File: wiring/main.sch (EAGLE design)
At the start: 38 parts, among them IC1 attiny 2313A, J2 J7MM, J3 J5MM, J4 J10MM, J5 J7MM, J6 J5MM, J7 J5MM, Q1 12MHz, T1 BD433, X1 USB-B

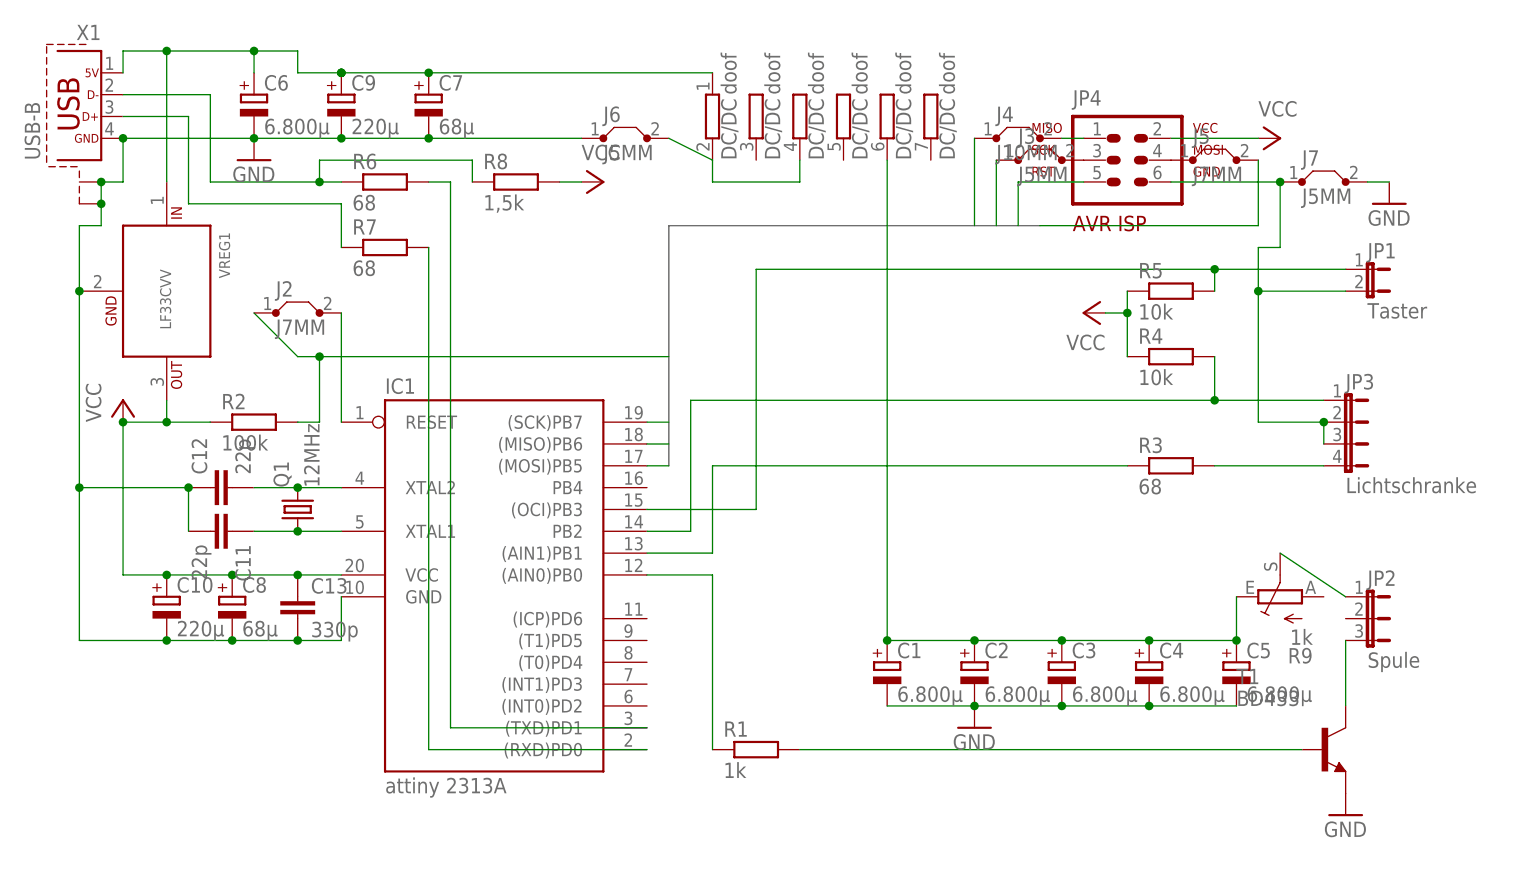
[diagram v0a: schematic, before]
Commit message: ändern auf mosfet
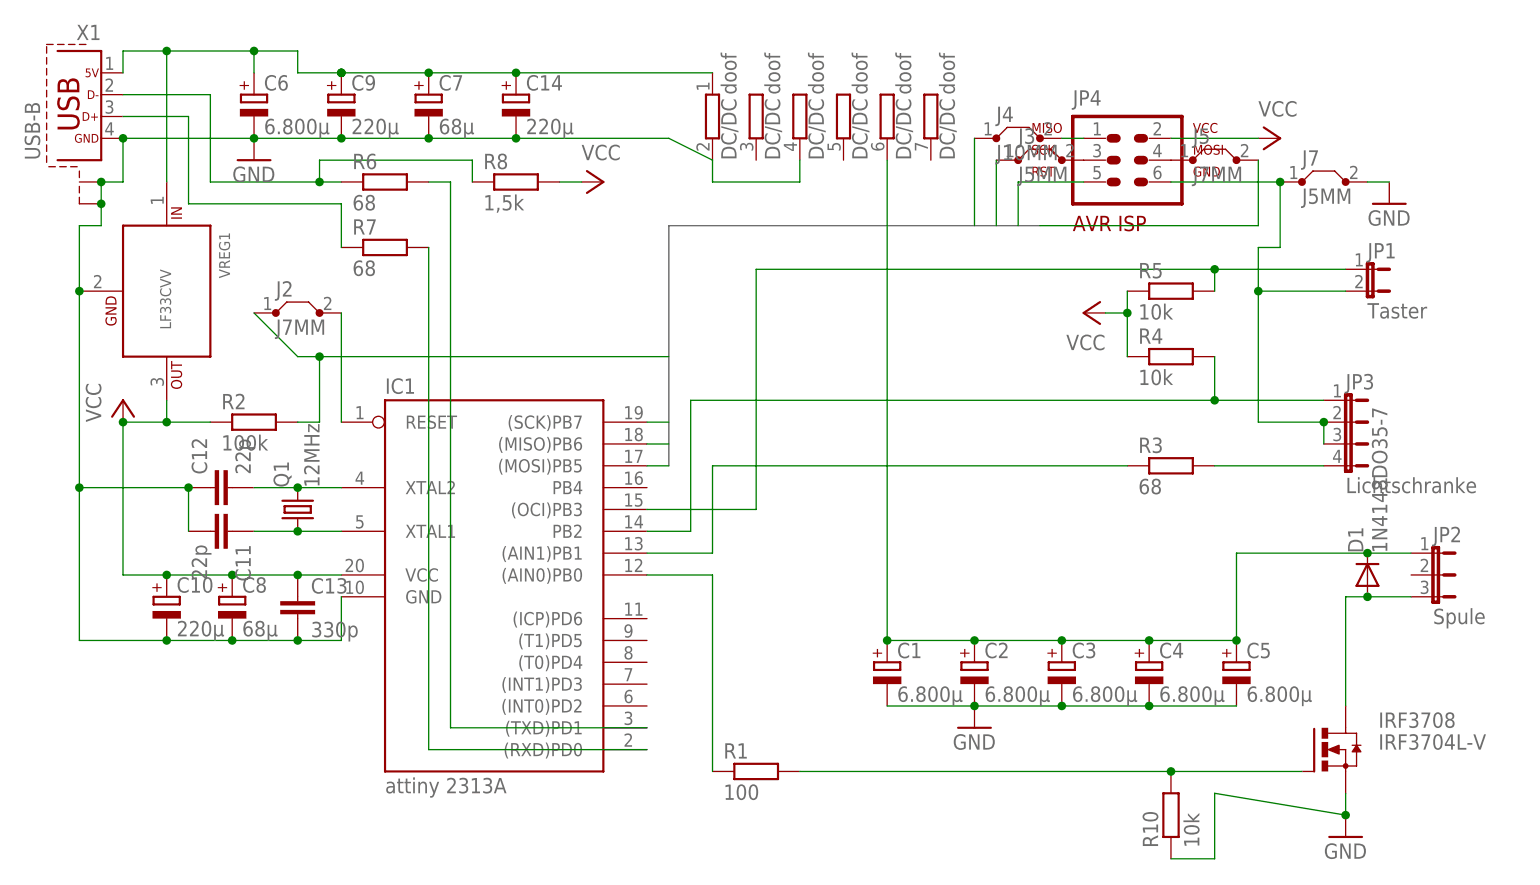
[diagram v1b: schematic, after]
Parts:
- removed J6: J5MM, jumper:J5MM
- removed R9: 1k, pot:TRIM_EU-PT10
- removed T1: BD433, transistor:BD239
- added C14: 220µ, resistor:CPOL-EUE2.5-7
- added D1: 1N4148DO35-7, diode:1N4148DO35-7
- added IRF3708: IRF3704L-V, transistor-power:IRF3704L-V
- added R10: 10k, rcl:R-EU_0207/10
- R1: value 1k -> 100
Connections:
- removed net N$21: DC/DCA.2, DC/DCC.2, J6.2
- removed net N$5: JP2.1, R9.S
- net 5V: now also C14.+
- net GND: now also C14.-, DC/DCA.2, DC/DCC.2, IRF3708.S, R10.1; no longer J6.1, T1.E
- net N$2: now also IRF3708.G, R10.2; no longer T1.B
- net N$3: now also D1.A, IRF3708.D; no longer T1.C
- net N$4: now also D1.C, JP2.1; no longer R9.E
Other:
- moved on the sheet: JP2, R1
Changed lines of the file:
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@@
 <part name="C9" library="resistor" deviceset="CPOL-EU" device="E2.5-7" value="220µ"/>
 <part name="C10" library="resistor" deviceset="CPOL-EU" device="E2.5-7" value="220µ"/>
-<part name="T1" library="transistor" deviceset="BD239" device="" value="BD433"/>
-<part name="R1" library="rcl" deviceset="R-EU_" device="0207/10" value="1k"/>
+<part name="R1" library="rcl" deviceset="R-EU_" device="0207/10" value="100"/>
 <part name="DC/DC" library="resistor-sil" deviceset="GE06RP" device="" value="doof"/>
 <part name="R2" library="rcl" deviceset="R-EU_" device="0207/10" value="100k"/>
@@
 <part name="P+1" library="supply1" deviceset="VCC" device=""/>
 <part name="GND6" library="supply1" deviceset="GND" device=""/>
-<part name="R9" library="pot" deviceset="TRIM_EU-" device="PT10" value="1k"/>
 <part name="J2" library="jumper" deviceset="J" device="7MM" value="J7MM"/>
 <part name="GND7" library="supply1" deviceset="GND" device=""/>
@@
 <part name="J4" library="jumper" deviceset="J" device="10MM"/>
 <part name="J5" library="jumper" deviceset="J" device="7MM" value="J7MM"/>
-<part name="J6" library="jumper" deviceset="J" device="5MM"/>
 <part name="GND4" library="supply1" deviceset="GND" device=""/>
 <part name="J7" library="jumper" deviceset="J" device="5MM"/>
 <part name="GND3" library="supply1" deviceset="GND" device=""/>
+<part name="D1" library="diode" deviceset="1N4148" device="DO35-7"/>
+<part name="IRF3708" library="transistor-power" deviceset="IRF3704" device="L-V"/>
+<part name="R10" library="rcl" deviceset="R-EU_" device="0207/10" value="10k"/>
+<part name="C14" library="resistor" deviceset="CPOL-EU" device="E2.5-7" value="220µ"/>
 </parts>
 <sheets>
@@
 <instance part="IC1" gate="G$1" x="25.4" y="33.02"/>
 <instance part="JP1" gate="A" x="127" y="71.12" rot="R270"/>
-<instance part="JP2" gate="1" x="127" y="30.48" rot="R270"/>
+<instance part="JP2" gate="1" x="134.62" y="35.56" rot="R270"/>
 <instance part="JP3" gate="G$1" x="124.46" y="53.34" rot="R270"/>
 <instance part="C1" gate="G$1" x="71.12" y="25.4"/>
@@
 <instance part="C9" gate="G$1" x="7.62" y="91.44"/>
 <instance part="C10" gate="G$1" x="-12.7" y="33.02"/>
-<instance part="T1" gate="G$1" x="121.92" y="15.24"/>
-<instance part="R1" gate="G$1" x="55.88" y="15.24"/>
+<instance part="R1" gate="G$1" x="55.88" y="12.7"/>
 <instance part="DC/DC" gate="A" x="50.8" y="88.9"/>
 <instance part="DC/DC" gate="B" x="55.88" y="88.9"/>
@@
 <instance part="P+4" gate="VCC" x="116.84" y="86.36" rot="R270"/>
 <instance part="P+1" gate="VCC" x="-17.78" y="55.88"/>
-<instance part="GND6" gate="1" x="124.46" y="7.62"/>
-<instance part="R9" gate="1" x="116.84" y="33.02" rot="R90"/>
+<instance part="GND6" gate="1" x="124.46" y="5.08"/>
 <instance part="J2" gate="1" x="2.54" y="66.04"/>
 <instance part="GND7" gate="1" x="129.54" y="78.74"/>
@@
 <instance part="J4" gate="1" x="86.36" y="86.36"/>
 <instance part="J5" gate="1" x="109.22" y="83.82"/>
-<instance part="J6" gate="1" x="40.64" y="86.36"/>
 <instance part="GND4" gate="1" x="81.28" y="17.78"/>
 <instance part="J7" gate="1" x="121.92" y="81.28"/>
 <instance part="GND3" gate="1" x="-2.54" y="83.82"/>
+<instance part="D1" gate="G$1" x="127" y="35.56" rot="R90"/>
+<instance part="IRF3708" gate="G$1" x="121.92" y="15.24"/>
+<instance part="R10" gate="G$1" x="104.14" y="7.62" rot="R90"/>
+<instance part="C14" gate="G$1" x="27.94" y="91.44"/>
 </instances>
 <busses>
@@
 <segment>
 <pinref part="R1" gate="G$1" pin="2"/>
-<pinref part="T1" gate="G$1" pin="B"/>
-<wire x1="60.96" y1="15.24" x2="119.38" y2="15.24" width="0.1524" layer="91"/>
+<wire x1="60.96" y1="12.7" x2="104.14" y2="12.7" width="0.1524" layer="91"/>
+<pinref part="R10" gate="G$1" pin="2"/>
+<pinref part="IRF3708" gate="G$1" pin="G"/>
+<wire x1="104.14" y1="12.7" x2="119.38" y2="12.7" width="0.1524" layer="91"/>
+<junction x="104.14" y="12.7"/>
 </segment>
 </net>
@@
 <junction x="101.6" y="27.94"/>
 <junction x="91.44" y="27.94"/>
-<pinref part="R9" gate="1" pin="E"/>
-<wire x1="111.76" y1="27.94" x2="111.76" y2="33.02" width="0.1524" layer="91"/>
 <junction x="111.76" y="27.94"/>
+<wire x1="111.76" y1="27.94" x2="111.76" y2="38.1" width="0.1524" layer="91"/>
+<pinref part="JP2" gate="1" pin="1"/>
+<wire x1="111.76" y1="38.1" x2="127" y2="38.1" width="0.1524" layer="91"/>
+<pinref part="D1" gate="G$1" pin="C"/>
+<wire x1="127" y1="38.1" x2="132.08" y2="38.1" width="0.1524" layer="91"/>
+<junction x="127" y="38.1"/>
 </segment>
 </net>
@@
 <wire x1="7.62" y1="93.98" x2="17.78" y2="93.98" width="0.1524" layer="91"/>
 <pinref part="DC/DC" gate="A" pin="1"/>
-<wire x1="17.78" y1="93.98" x2="50.8" y2="93.98" width="0.1524" layer="91"/>
+<wire x1="17.78" y1="93.98" x2="27.94" y2="93.98" width="0.1524" layer="91"/>
 <junction x="7.62" y="93.98"/>
 <junction x="17.78" y="93.98"/>
 <junction x="7.62" y="93.98"/>
+<wire x1="27.94" y1="93.98" x2="50.8" y2="93.98" width="0.1524" layer="91"/>
 <wire x1="7.62" y1="93.98" x2="2.54" y2="93.98" width="0.1524" layer="91"/>
 <wire x1="2.54" y1="93.98" x2="2.54" y2="96.52" width="0.1524" layer="91"/>
@@
 <wire x1="-2.54" y1="93.98" x2="-2.54" y2="96.52" width="0.1524" layer="91"/>
 <junction x="-2.54" y="96.52"/>
+<pinref part="C14" gate="G$1" pin="+"/>
+<junction x="27.94" y="93.98"/>
 </segment>
 </net>
@@
 <segment>
 <pinref part="R1" gate="G$1" pin="1"/>
-<wire x1="50.8" y1="15.24" x2="50.8" y2="35.56" width="0.1524" layer="91"/>
+<wire x1="50.8" y1="12.7" x2="50.8" y2="35.56" width="0.1524" layer="91"/>
 <pinref part="IC1" gate="G$1" pin="(AIN0)PB0"/>
 <wire x1="50.8" y1="35.56" x2="43.18" y2="35.56" width="0.1524" layer="91"/>
@@
 <pinref part="C7" gate="G$1" pin="-"/>
 <wire x1="7.62" y1="86.36" x2="17.78" y2="86.36" width="0.1524" layer="91"/>
-<wire x1="17.78" y1="86.36" x2="35.56" y2="86.36" width="0.1524" layer="91"/>
+<wire x1="17.78" y1="86.36" x2="27.94" y2="86.36" width="0.1524" layer="91"/>
 <junction x="-2.54" y="86.36"/>
 <junction x="7.62" y="86.36"/>
 <junction x="17.78" y="86.36"/>
+<wire x1="27.94" y1="86.36" x2="45.72" y2="86.36" width="0.1524" layer="91"/>
 <wire x1="-17.78" y1="86.36" x2="-17.78" y2="81.28" width="0.1524" layer="91"/>
 <pinref part="X1" gate="G$1" pin="S1"/>
@@
 <junction x="-20.32" y="81.28"/>
 <junction x="-17.78" y="86.36"/>
-<pinref part="J6" gate="1" pin="1"/>
 <pinref part="GND3" gate="1" pin="GND"/>
 <pinref part="C12" gate="G$1" pin="1"/>
@@
 <junction x="-12.7" y="27.94"/>
 <junction x="-22.86" y="45.72"/>
-</segment>
-<segment>
-<pinref part="T1" gate="G$1" pin="E"/>
-<pinref part="GND6" gate="1" pin="GND"/>
+<pinref part="DC/DC" gate="A" pin="2"/>
+<wire x1="45.72" y1="86.36" x2="50.8" y2="83.82" width="0.1524" layer="91"/>
+<wire x1="50.8" y1="83.82" x2="50.8" y2="81.28" width="0.1524" layer="91"/>
+<wire x1="50.8" y1="81.28" x2="60.96" y2="81.28" width="0.1524" layer="91"/>
+<pinref part="DC/DC" gate="C" pin="2"/>
+<wire x1="60.96" y1="81.28" x2="60.96" y2="83.82" width="0.1524" layer="91"/>
+<pinref part="C14" gate="G$1" pin="-"/>
+<junction x="27.94" y="86.36"/>
 </segment>
 <segment>
@@
 <pinref part="GND4" gate="1" pin="GND"/>
 </segment>
+<segment>
+<pinref part="GND6" gate="1" pin="GND"/>
+<pinref part="IRF3708" gate="G$1" pin="S"/>
+<wire x1="124.46" y1="7.62" x2="109.22" y2="10.16" width="0.1524" layer="91"/>
+<wire x1="109.22" y1="10.16" x2="109.22" y2="2.54" width="0.1524" layer="91"/>
+<pinref part="R10" gate="G$1" pin="1"/>
+<wire x1="109.22" y1="2.54" x2="104.14" y2="2.54" width="0.1524" layer="91"/>
+<junction x="124.46" y="7.62"/>
+<wire x1="124.46" y1="7.62" x2="124.46" y2="10.16" width="0.1524" layer="91"/>
+</segment>
 </net>
 <net name="SCK" class="0">
@@
 </segment>
 </net>
-<net name="N$5" class="0">
-<segment>
-<pinref part="R9" gate="1" pin="S"/>
-<pinref part="JP2" gate="1" pin="1"/>
-<wire x1="116.84" y1="38.1" x2="124.46" y2="33.02" width="0.1524" layer="91"/>
-</segment>
-</net>
 <net name="N$7" class="0">
 <segment>
@@
 </segment>
 </net>
-<net name="N$21" class="0">
-<segment>
-<pinref part="DC/DC" gate="A" pin="2"/>
-<wire x1="45.72" y1="86.36" x2="50.8" y2="83.82" width="0.1524" layer="91"/>
-<pinref part="J6" gate="1" pin="2"/>
-<wire x1="50.8" y1="83.82" x2="50.8" y2="81.28" width="0.1524" layer="91"/>
-<wire x1="50.8" y1="81.28" x2="60.96" y2="81.28" width="0.1524" layer="91"/>
-<pinref part="DC/DC" gate="C" pin="2"/>
-<wire x1="60.96" y1="81.28" x2="60.96" y2="83.82" width="0.1524" layer="91"/>
-</segment>
-</net>
 <net name="N$3" class="0">
 <segment>
 <pinref part="JP2" gate="1" pin="3"/>
-<wire x1="124.46" y1="27.94" x2="124.46" y2="20.32" width="0.1524" layer="91"/>
-<pinref part="T1" gate="G$1" pin="C"/>
-</segment>
-</net>
+<wire x1="132.08" y1="33.02" x2="127" y2="33.02" width="0.1524" layer="91"/>
+<wire x1="127" y1="33.02" x2="124.46" y2="33.02" width="0.1524" layer="91"/>
+<wire x1="124.46" y1="33.02" x2="124.46" y2="20.32" width="0.1524" layer="91"/>
+<pinref part="D1" gate="G$1" pin="A"/>
+<junction x="127" y="33.02"/>
+<pinref part="IRF3708" gate="G$1" pin="D"/>
+</segment>
+</net>

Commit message: zwischenspeichern schaltplan schöner zeichnen
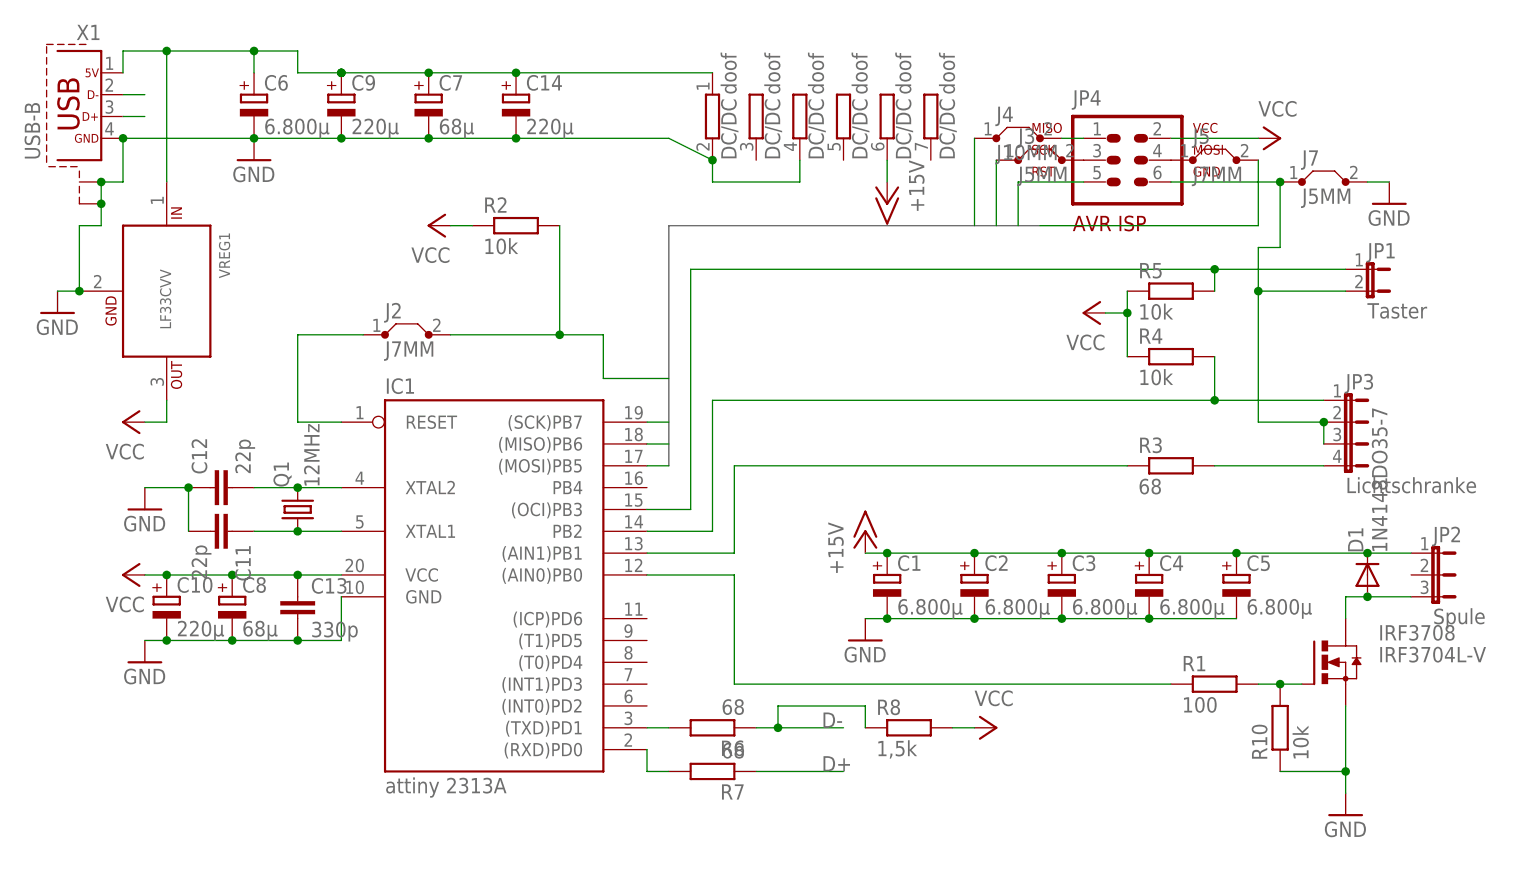
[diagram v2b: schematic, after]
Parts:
- R2: value 100k -> 10k
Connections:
- net N$1 renamed PB0
- net N$16 renamed D-
- net N$17 renamed D+
- net N$4 renamed +15V
- removed net N$7: IC1.RESET, J2.2
- removed net RST: J2.1, JP4.5, R2.2
- new net N$1: IC1.RESET, J2.1
- new net RST1: J2.2, JP4.5, R2.2
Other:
- moved on the sheet: C1, C2, C3, C4, C5, IRF3708, J2, R1, R10, R2, R6, R7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
